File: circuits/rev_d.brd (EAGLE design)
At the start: 80.8 x 49 mm, 16 parts, among them X1 ENCODER_ANO

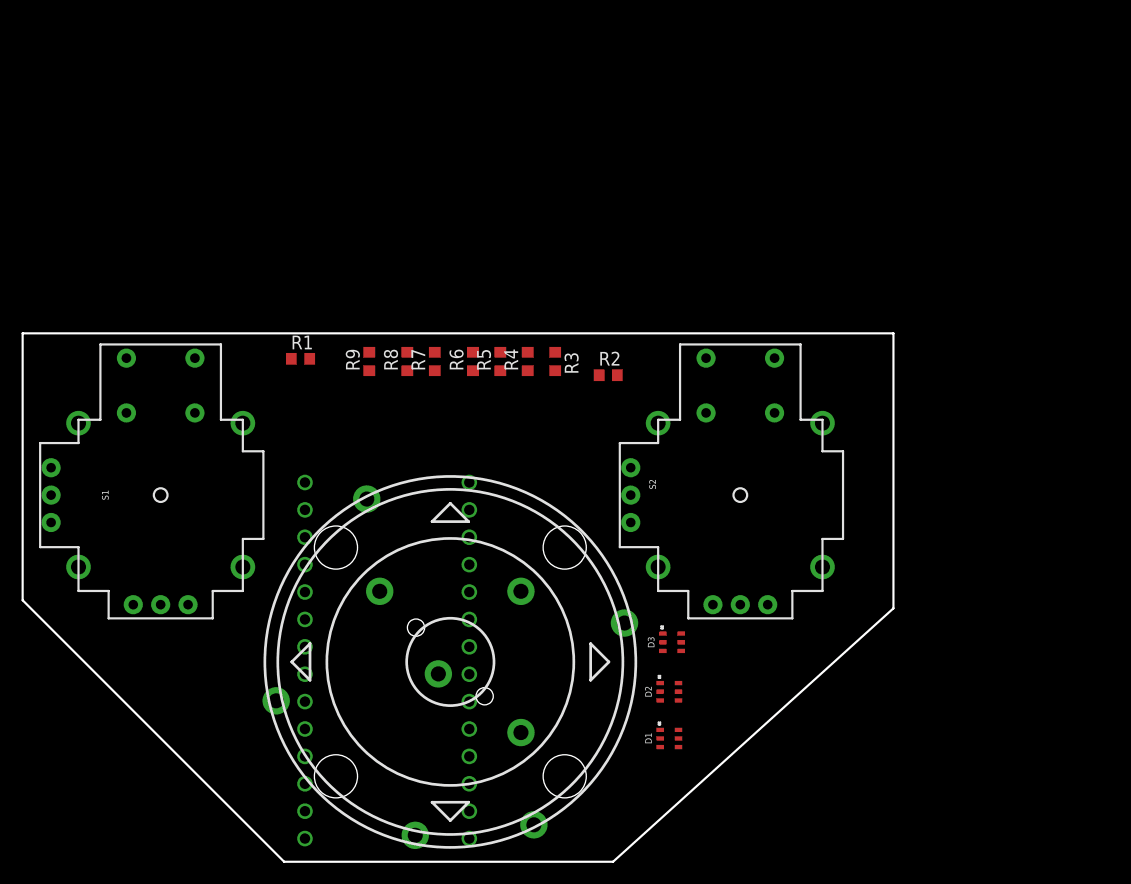
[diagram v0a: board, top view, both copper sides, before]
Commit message: Trying again on the circuit, fiddling with settings for nice scrolling in eagle.
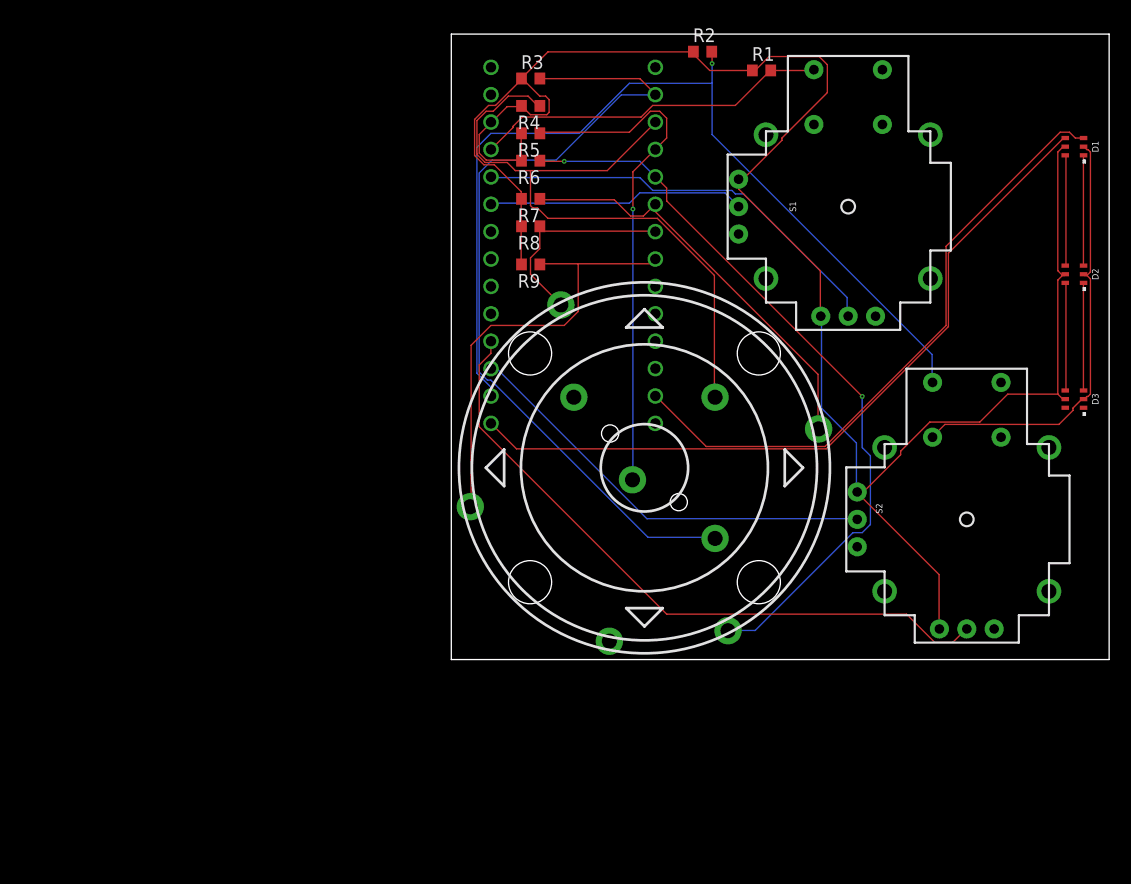
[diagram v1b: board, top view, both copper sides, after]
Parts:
- moved S1 69.1 mm to (36.8, 42.0)
- moved D1 66.5 mm to (57.8, 47.6), turned to 270 degrees
- moved D2 53.9 mm to (57.8, 35.7), turned to 270 degrees
- moved R1 50.4 mm to (28.8, 54.6)
- moved D3 43.6 mm to (57.8, 24.1), turned to 270 degrees
- moved MCU 42.2 mm to (11.3, 38.4)
- moved R2 31.2 mm to (23.3, 56.4)
- moved R3 26.3 mm to (7.36, 53.9), turned to 0 degrees
- moved X1 25.5 mm to (17.9, 17.8)
- moved R4 23.7 mm to (7.36, 51.3), turned to 180 degrees
- moved R5 21.3 mm to (7.36, 48.8), turned to 180 degrees
- moved S2 21.1 mm to (47.8, 13.0)
- moved R6 19.4 mm to (7.36, 46.3), turned to 180 degrees
- moved R7 17.5 mm to (7.36, 42.7), turned to 180 degrees
- moved R9 17.5 mm to (7.36, 36.6), turned to 180 degrees
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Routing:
- net +3V3: track 0.00 -> 185.8 mm
- net S2: track 0.00 -> 87.0 mm, vias 0 -> 1
- net N$7: track 0.00 -> 77.4 mm
- net N$12: track 0.00 -> 70.2 mm
- net N$4: track 0.00 -> 69.1 mm, vias 0 -> 2
- net N$6: track 0.00 -> 63.7 mm
- net HOR2: track 0.00 -> 62.4 mm
- net N$13: track 0.00 -> 58.2 mm
- net N$5: track 0.00 -> 47.7 mm, vias 0 -> 1
- net N$1: track 0.00 -> 41.6 mm
- net GND: track 0.00 -> 40.7 mm
- net VERT2: track 0.00 -> 39.7 mm
- net HOR1: track 0.00 -> 39.5 mm
- net N$3: track 0.00 -> 39.2 mm
- net S1: track 0.00 -> 33.1 mm
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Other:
- board size 80.8 x 49 mm -> 61 x 58 mm
